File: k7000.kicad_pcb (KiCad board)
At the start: 2 copper layers, 61 x 43.2 mm, 7 parts, among them J1 Conn_01x13

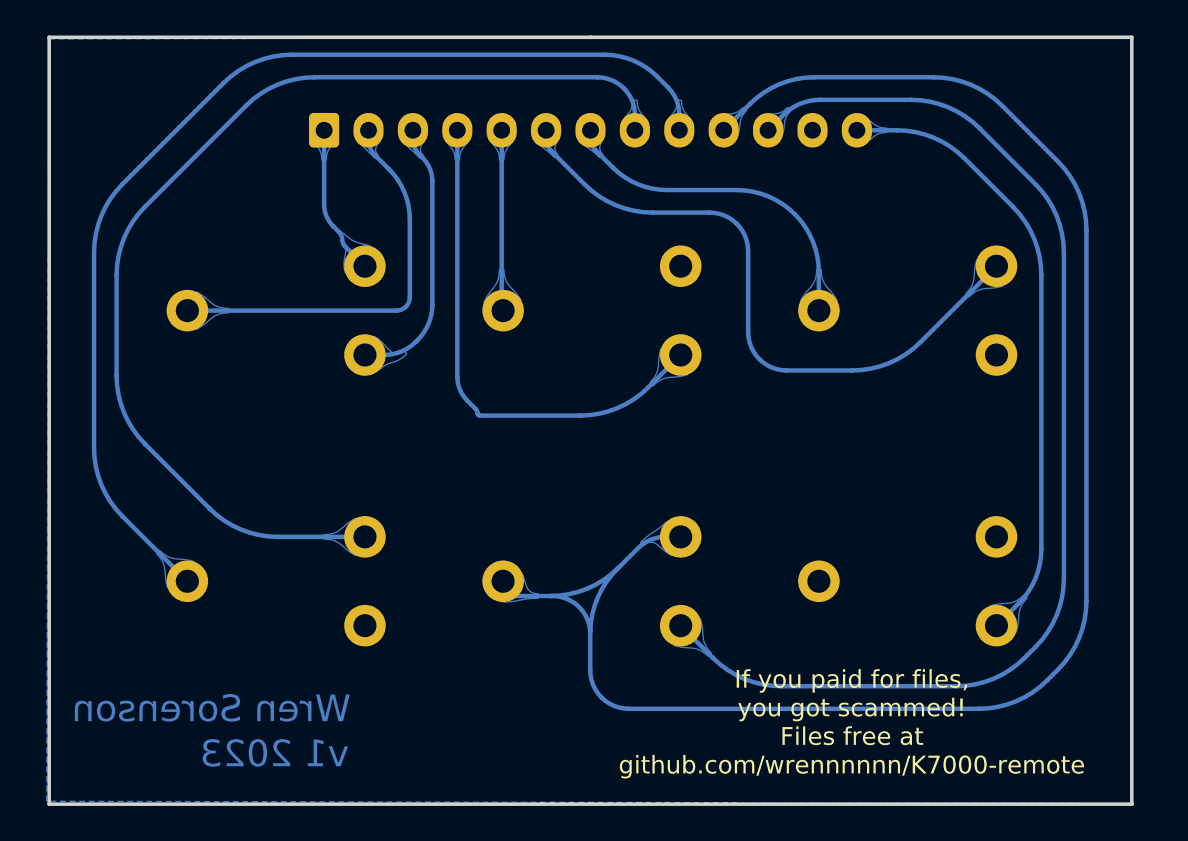
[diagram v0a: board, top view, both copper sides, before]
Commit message: fixed issues
added silkscreen
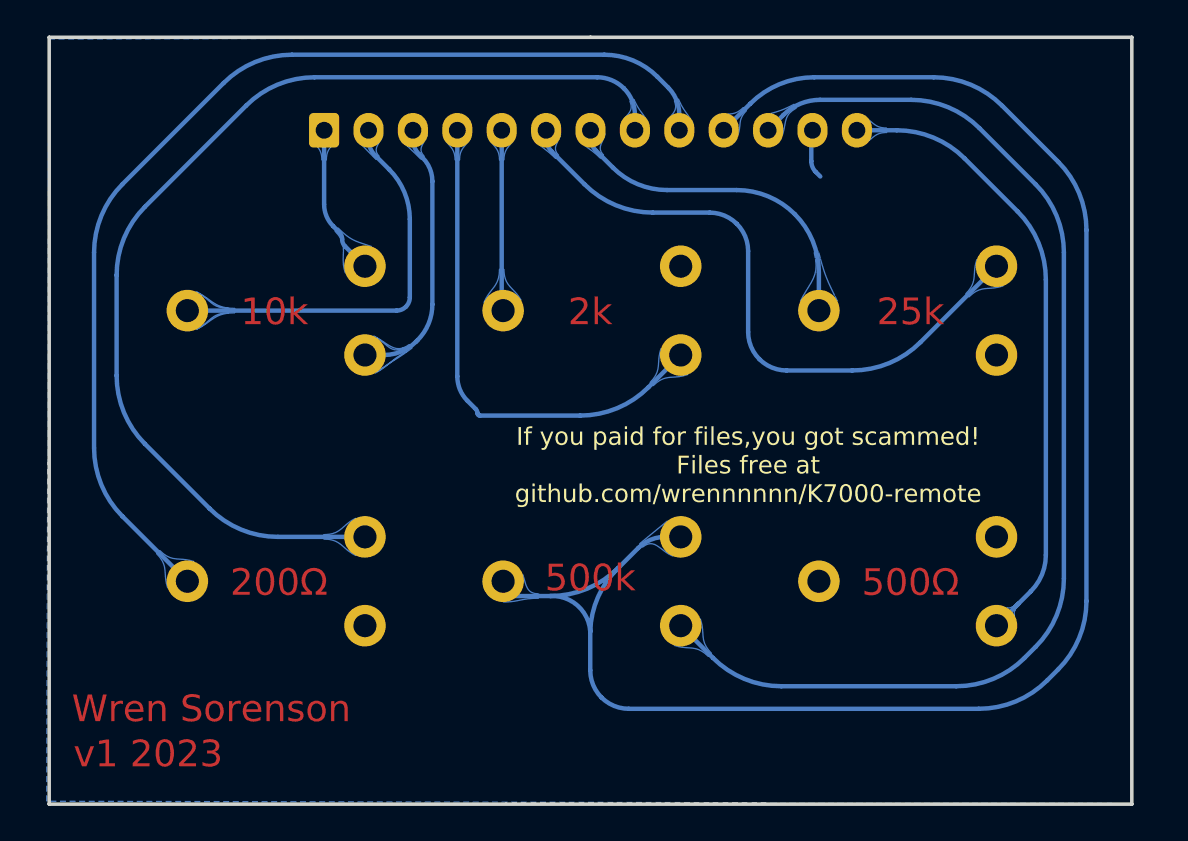
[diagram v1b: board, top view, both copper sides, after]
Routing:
- net Net-(RV2-Pad1): track 0.00 -> 2.80 mm
- net Net-(RV6-Pad1): track 35.1 -> 35.8 mm
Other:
- board text added: "10k"
- board text added: "200Ω"
- board text added: "25k"
- board text added: "2k"
- board text added: "500k"
- board text added: "500Ω"
- board text added: "BLK LEVEL"
- board text added: "CONTRAST"
- board text added: "H-POS"
- board text added: "If you paid for files,you got scammed! Files free at github.com/wrennnnnn/K7000-remote"
- board text added: "V-HOLD"
- board text added: "V-POS"
- board text added: "V-SIZE"
- board text removed: "If you paid for files, you got scammed! Files free at github.com/wrennnnnn/K7000-remote"
